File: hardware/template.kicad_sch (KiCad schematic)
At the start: 0 parts

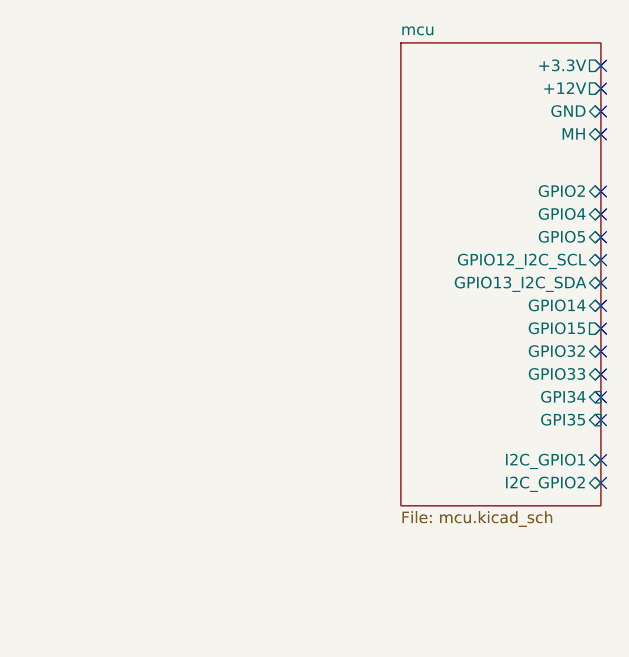
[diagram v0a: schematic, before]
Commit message: new
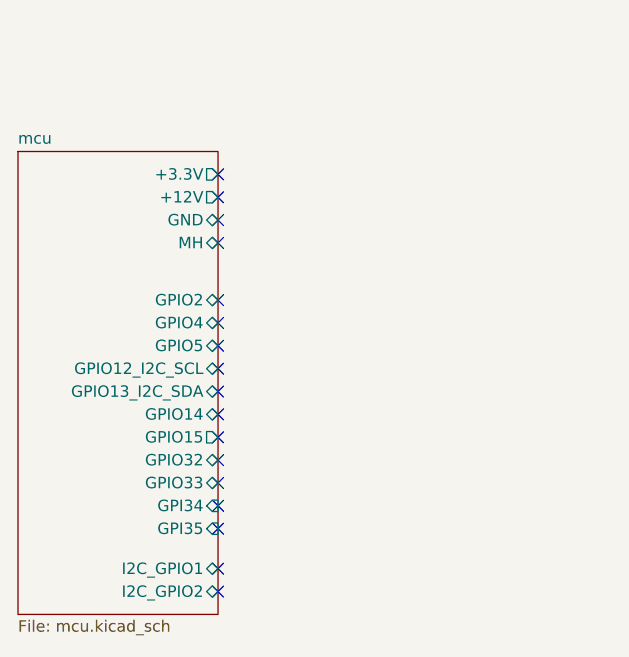
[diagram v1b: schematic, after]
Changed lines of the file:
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@@
 (kicad_sch (version 20230121) (generator eeschema)
   (paper "A4")
-  (no_connect (at 138.43 76.2))
-  (no_connect (at 138.43 88.9))
-  (no_connect (at 138.43 91.44))
-  (no_connect (at 138.43 93.98))
-  (no_connect (at 138.43 96.52))
-  (no_connect (at 138.43 78.74))
-  (no_connect (at 138.43 81.28))
-  (no_connect (at 138.43 83.82))
-  (no_connect (at 138.43 86.36))
-  (no_connect (at 138.43 71.12))
-  (no_connect (at 138.43 59.69))
-  (no_connect (at 138.43 62.23))
-  (no_connect (at 138.43 103.505))
-  (no_connect (at 138.43 57.15))
-  (no_connect (at 138.43 73.66))
-  (no_connect (at 138.43 64.77))
-  (no_connect (at 138.43 100.965))
-  (sheet (at 116.205 54.61) (size 22.225 51.435) (fields_autoplaced)
+  (no_connect (at 95.885 88.265))
+  (no_connect (at 95.885 100.965))
+  (no_connect (at 95.885 103.505))
+  (no_connect (at 95.885 106.045))
+  (no_connect (at 95.885 108.585))
+  (no_connect (at 95.885 90.805))
+  (no_connect (at 95.885 93.345))
+  (no_connect (at 95.885 95.885))
+  (no_connect (at 95.885 98.425))
+  (no_connect (at 95.885 83.185))
+  (no_connect (at 95.885 71.755))
+  (no_connect (at 95.885 74.295))
+  (no_connect (at 95.885 115.57))
+  (no_connect (at 95.885 69.215))
+  (no_connect (at 95.885 85.725))
+  (no_connect (at 95.885 76.835))
+  (no_connect (at 95.885 113.03))
+  (sheet (at 73.66 66.675) (size 22.225 51.435) (fields_autoplaced)
     (stroke (width 0) (type solid))
     (fill (color 0 0 0 0.0000))
-    (property "Sheetname" "mcu" (at 116.205 53.8984 0)
+    (property "Sheetname" "mcu" (at 73.66 65.9634 0)
       (effects (font (size 1.27 1.27)) (justify left bottom))
     )
-    (property "Sheetfile" "mcu.kicad_sch" (at 116.205 106.6296 0)
+    (property "Sheetfile" "mcu.kicad_sch" (at 73.66 118.6946 0)
       (effects (font (size 1.27 1.27)) (justify left top))
     )
-    (pin "GPIO2" bidirectional (at 138.43 71.12 0)
+    (pin "GPIO2" bidirectional (at 95.885 83.185 0)
       (effects (font (size 1.27 1.27)) (justify right))
     )
-    (pin "GPIO13_I2C_SDA" bidirectional (at 138.43 81.28 0)
+    (pin "GPIO13_I2C_SDA" bidirectional (at 95.885 93.345 0)
       (effects (font (size 1.27 1.27)) (justify right))
     )
-    (pin "GPIO14" bidirectional (at 138.43 83.82 0)
+    (pin "GPIO14" bidirectional (at 95.885 95.885 0)
       (effects (font (size 1.27 1.27)) (justify right))
     )
-    (pin "GPIO15" output (at 138.43 86.36 0)
+    (pin "GPIO15" output (at 95.885 98.425 0)
       (effects (font (size 1.27 1.27)) (justify right))
     )
-    (pin "GPIO32" bidirectional (at 138.43 88.9 0)
+    (pin "GPIO32" bidirectional (at 95.885 100.965 0)
       (effects (font (size 1.27 1.27)) (justify right))
     )
-    (pin "+12V" output (at 138.43 59.69 0)
+    (pin "+12V" output (at 95.885 71.755 0)
       (effects (font (size 1.27 1.27)) (justify right))
     )
-    (pin "+3.3V" output (at 138.43 57.15 0)
+    (pin "+3.3V" output (at 95.885 69.215 0)
       (effects (font (size 1.27 1.27)) (justify right))
     )
-    (pin "GND" bidirectional (at 138.43 62.23 0)
+    (pin "GND" bidirectional (at 95.885 74.295 0)
       (effects (font (size 1.27 1.27)) (justify right))
     )
-    (pin "GPI34" input (at 138.43 93.98 0)
+    (pin "GPI34" input (at 95.885 106.045 0)
       (effects (font (size 1.27 1.27)) (justify right))
     )
-    (pin "GPI35" input (at 138.43 96.52 0)
+    (pin "GPI35" input (at 95.885 108.585 0)
       (effects (font (size 1.27 1.27)) (justify right))
     )
-    (pin "GPIO33" bidirectional (at 138.43 91.44 0)
+    (pin "GPIO33" bidirectional (at 95.885 103.505 0)
       (effects (font (size 1.27 1.27)) (justify right))
     )
-    (pin "GPIO12_I2C_SCL" bidirectional (at 138.43 78.74 0)
+    (pin "GPIO12_I2C_SCL" bidirectional (at 95.885 90.805 0)
       (effects (font (size 1.27 1.27)) (justify right))
     )
-    (pin "MH" bidirectional (at 138.43 64.77 0)
+    (pin "MH" bidirectional (at 95.885 76.835 0)
       (effects (font (size 1.27 1.27)) (justify right))
     )
-    (pin "GPIO5" bidirectional (at 138.43 76.2 0)
+    (pin "GPIO5" bidirectional (at 95.885 88.265 0)
       (effects (font (size 1.27 1.27)) (justify right))
     )
-    (pin "GPIO4" bidirectional (at 138.43 73.66 0)
+    (pin "GPIO4" bidirectional (at 95.885 85.725 0)
       (effects (font (size 1.27 1.27)) (justify right))
     )
-    (pin "I2C_GPIO2" bidirectional (at 138.43 103.505 0)
+    (pin "I2C_GPIO2" bidirectional (at 95.885 115.57 0)
       (effects (font (size 1.27 1.27)) (justify right))
     )
-    (pin "I2C_GPIO1" bidirectional (at 138.43 100.965 0)
+    (pin "I2C_GPIO1" bidirectional (at 95.885 113.03 0)
       (effects (font (size 1.27 1.27)) (justify right))
     )
